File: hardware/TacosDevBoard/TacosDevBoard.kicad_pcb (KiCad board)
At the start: 2 copper layers, 39.1 x 59.4 mm, 6 parts, among them J1 Conn_01x15_Socket, J2 Conn_01x15_Socket, J3 Conn_01x08_Socket, J4 Conn_01x08_Socket

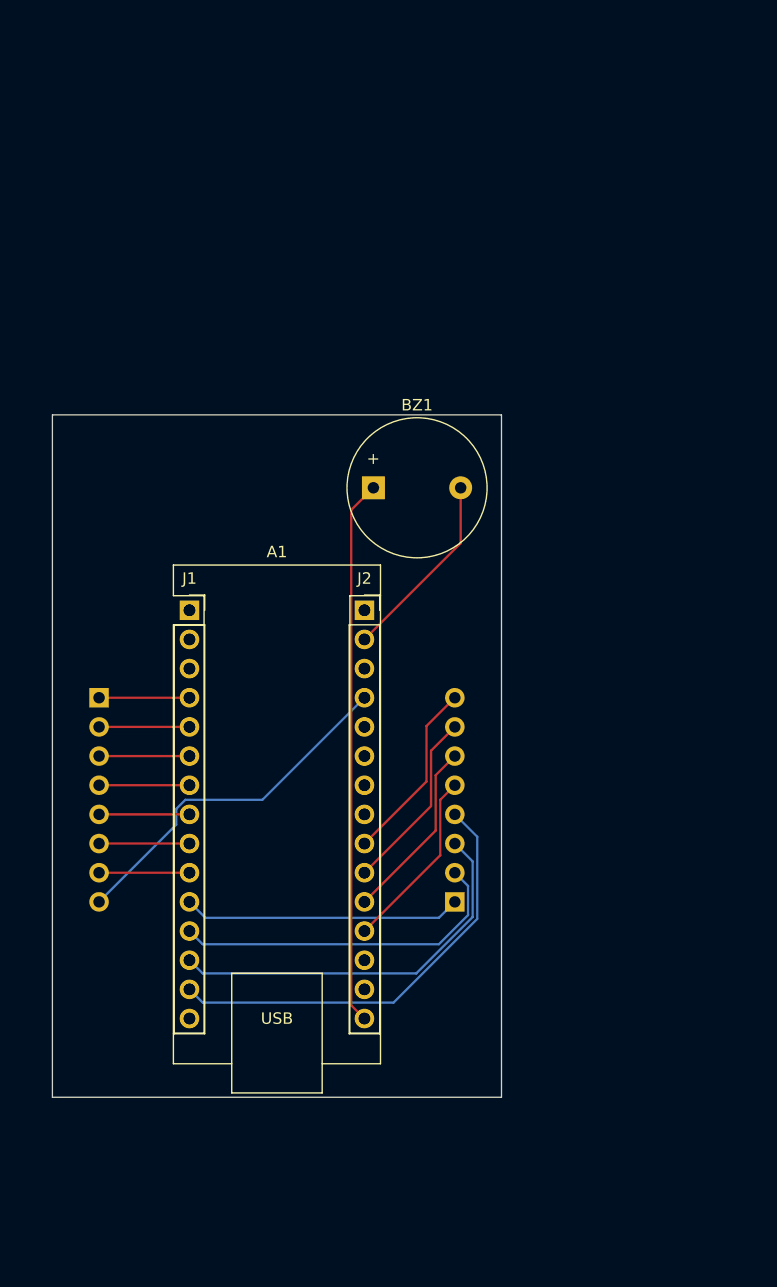
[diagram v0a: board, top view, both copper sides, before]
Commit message: finished mega pcb
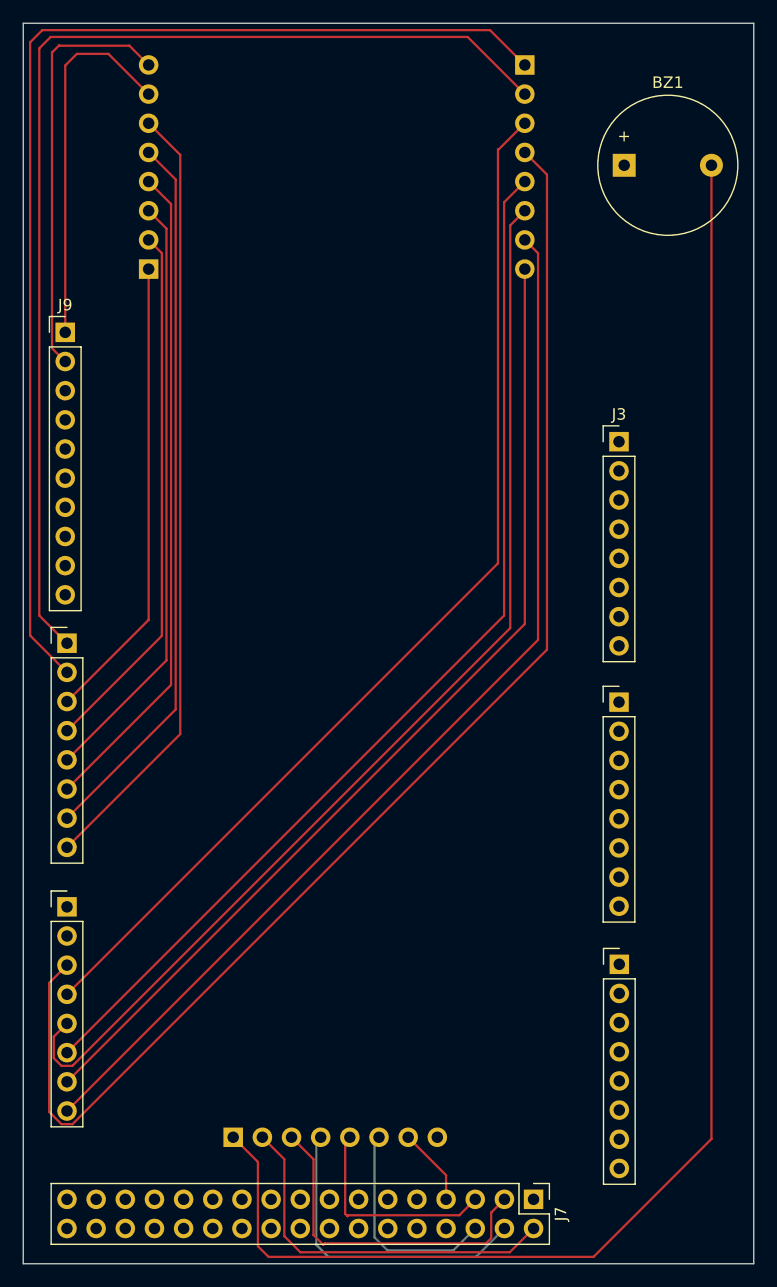
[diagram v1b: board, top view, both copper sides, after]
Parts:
- removed A1: Arduino_Nano_v3.x, Module:Arduino_Nano
- added IC2_COMM1: Conn_01x08_Socket, Connector_PinSocket_2.54mm:PinSocket_1x08_P2.54mm_Vertical, B.Cu at (152.9, 38.1)
- added J3: Conn_01x08_Socket, Connector_PinHeader_2.54mm:PinHeader_1x08_P2.54mm_Vertical, F.Cu at (161.1, 70.9)
- added J4: Conn_01x08_Socket, Connector_PinHeader_2.54mm:PinHeader_1x08_P2.54mm_Vertical, F.Cu at (113.0, 111.4)
- added J5: Conn_01x08_Socket, Connector_PinHeader_2.54mm:PinHeader_1x08_P2.54mm_Vertical, F.Cu at (113.0, 88.5)
- added J7: Conn_02x17_Counter_Clockwise, Connector_PinHeader_2.54mm:PinHeader_2x17_P2.54mm_Vertical, F.Cu at (153.7, 136.9)
- added J9: Conn_01x10_Pin, Connector_PinHeader_2.54mm:PinHeader_1x10_P2.54mm_Vertical, F.Cu at (112.9, 61.4)
- J1, J2: value Conn_01x15_Socket -> Conn_01x08_Socket; footprint Connector_PinSocket_2.54mm:PinSocket_1x15_P2.54mm_Vertical -> Connector_PinHeader_2.54mm:PinHeader_1x08_P2.54mm_Vertical
- moved PWM1 61.2 mm to (120.1, 55.9)
- moved J1 48.5 mm to (161.1, 116.4)
- moved SELECT1 40.0 mm to (127.5, 131.5), turned to -90 degrees
- moved BZ1 35.6 mm to (161.6, 46.8)
- moved J2 23.6 mm to (161.1, 93.6)
- renumbered J4 to PWM1, J3 to SELECT1
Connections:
- J1 pad 1: TX1 -> unconnected-(J1-Pin_1-Pad1)
- J1 pad 2: RX0 -> unconnected-(J1-Pin_2-Pad2)
- J1 pad 3: RST -> unconnected-(J1-Pin_3-Pad3)
- J1 pad 4: GND -> unconnected-(J1-Pin_4-Pad4)
- J1 pad 5: D2 -> unconnected-(J1-Pin_5-Pad5)
- J1 pad 6: D3 -> unconnected-(J1-Pin_6-Pad6)
- J1 pad 7: D4 -> unconnected-(J1-Pin_7-Pad7)
- J1 pad 8: D5 -> unconnected-(J1-Pin_8-Pad8)
- J2 pad 1: VIN -> unconnected-(J2-Pin_1-Pad1)
- J2 pad 2: GND -> unconnected-(J2-Pin_2-Pad2)
- J2 pad 3: RST -> unconnected-(J2-Pin_3-Pad3)
- J2 pad 4: +5V -> unconnected-(J2-Pin_4-Pad4)
- J2 pad 5: A7 -> unconnected-(J2-Pin_5-Pad5)
- J2 pad 6: A6 -> unconnected-(J2-Pin_6-Pad6)
- J2 pad 7: A5 -> unconnected-(J2-Pin_7-Pad7)
- J2 pad 8: A4 -> unconnected-(J2-Pin_8-Pad8)
- PWM1 pad 1: D8 -> ~D2
- PWM1 pad 2: D9 -> ~D3
- PWM1 pad 3: D10 -> ~D4
- PWM1 pad 4: D11 -> ~D5
- PWM1 pad 5: A0 -> ~D6
- PWM1 pad 6: A1 -> ~D7
- PWM1 pad 7: A2 -> ~D8
- PWM1 pad 8: A3 -> ~D9
- SELECT1 pad 2: D2 -> D22
- SELECT1 pad 3: D3 -> D24
- SELECT1 pad 4: D4 -> D26
- SELECT1 pad 5: D5 -> D28
- SELECT1 pad 6: D6 -> D30
- SELECT1 pad 7: D7 -> D32
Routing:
- net RX1: track 0.00 -> 118.5 mm
- net GND: track 24.6 -> 139.3 mm
- net TX0: track 0.00 -> 101.0 mm
- net RX0: track 0.00 -> 97.6 mm
- net RX2: track 0.00 -> 96.2 mm
- net TX3: track 0.00 -> 93.3 mm
- net TX1: track 0.00 -> 92.4 mm
- net TX2: track 0.00 -> 92.4 mm
- net RX3: track 0.00 -> 87.3 mm
- net ~D7: track 0.00 -> 68.3 mm
- net ~D6: track 0.00 -> 62.9 mm
- net ~D5: track 0.00 -> 57.5 mm
- net ~D4: track 0.00 -> 52.1 mm
- net D13: track 47.5 -> 0.00 mm
- net ~D3: track 0.00 -> 46.6 mm
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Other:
- board size 39.1 x 59.4 mm -> 63.6 x 108.1 mm
- board text added: "${REFERENCE}"
